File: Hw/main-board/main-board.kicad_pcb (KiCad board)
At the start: 2 copper layers, 93 x 45 mm, 33 parts, among them J1 AC_IN, J2 AC_OUT, J3 AC_OUT, K1 SRD-05VDC-SL-C, Q1 MMBT2222ALT1G, Q2 BTA12-600B, U1 LTV-354T, U2 Arduino-nano-BLE-33, U3 FODM3022, U4 SCD40-D-R2, U5 SGP40-D-R4

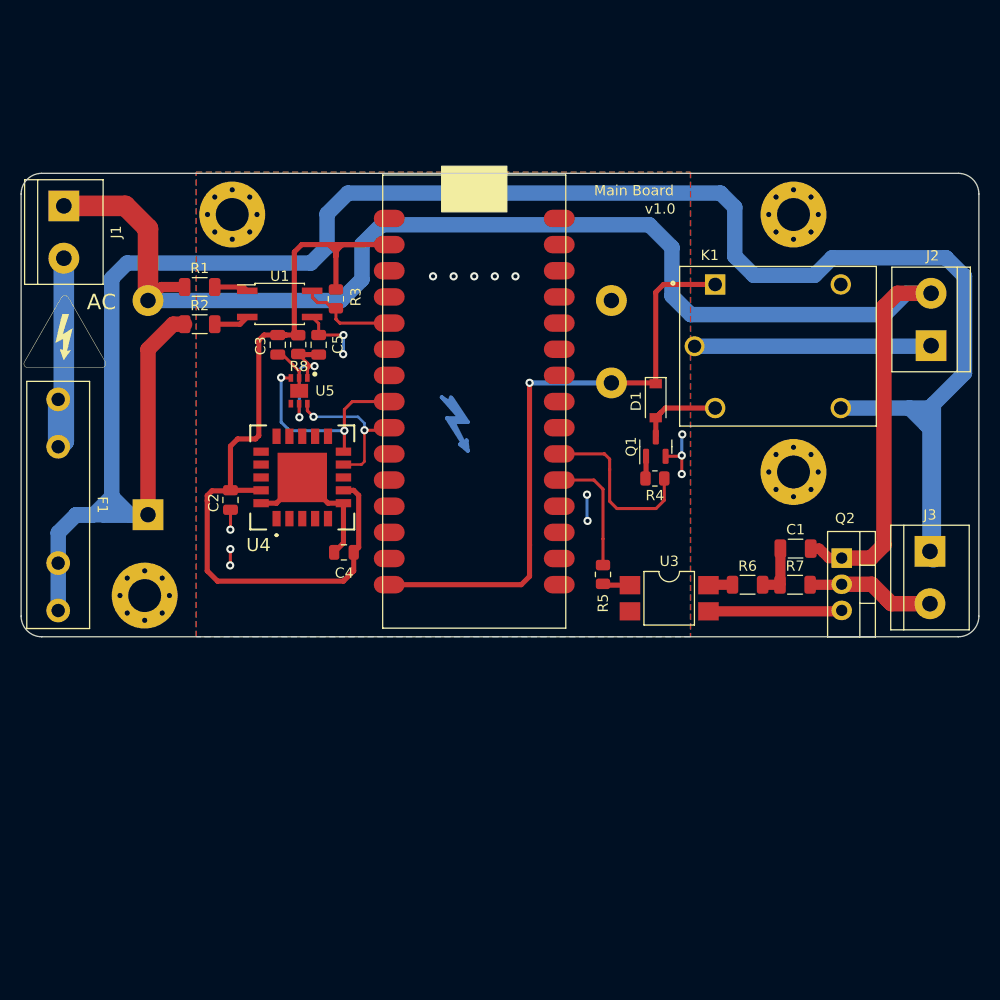
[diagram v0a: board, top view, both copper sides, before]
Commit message: update Kicad project
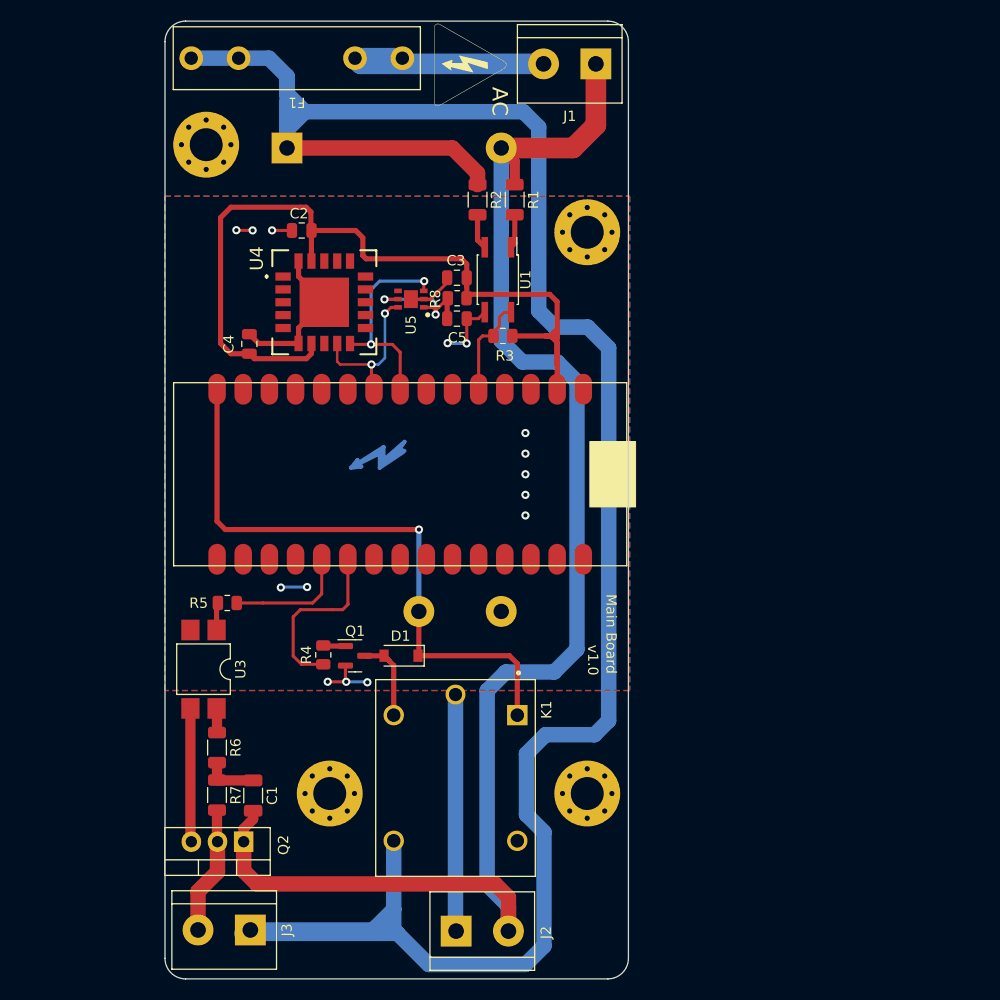
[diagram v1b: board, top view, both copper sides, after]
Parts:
- moved J3 75.5 mm to (90.3, 114.5), turned to 180 degrees
- moved J2 73.2 mm to (110.2, 114.6), turned to 0 degrees
- moved Q2 64.3 mm to (89.6, 105.9), turned to 180 degrees
- moved R7 59.7 mm to (87.0, 101.4), turned to -90 degrees
- moved REF** 59.7 mm to (123.0, 101.2), turned to -90 degrees
- moved C1 57.9 mm to (90.5, 101.4), turned to -90 degrees
- moved REF** 54.8 mm to (98.0, 101.2), turned to -90 degrees
- moved R6 53.9 mm to (87.0, 96.8), turned to -90 degrees
- moved J1 53.5 mm to (123.8, 30.4), turned to 180 degrees
- moved K1 52.3 mm to (110.2, 99.7), turned to -90 degrees
- moved G*** 47.1 mm to (111.6, 30.5), turned to -90 degrees
- moved F1 47.1 mm to (105.0, 29.8), turned to 180 degrees
- moved U3 45.7 mm to (85.7, 89.2), turned to -90 degrees
- moved REF** 44.2 mm to (86.0, 38.2), turned to -90 degrees
- moved PS1 38.1 mm to (93.8, 38.5), turned to -90 degrees
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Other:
- board size 93 x 45 mm -> 45 x 93 mm
